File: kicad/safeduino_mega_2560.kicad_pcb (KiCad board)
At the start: 4 copper layers, 134.5 x 63.9 mm, 108 parts, among them X1 USBB-1J

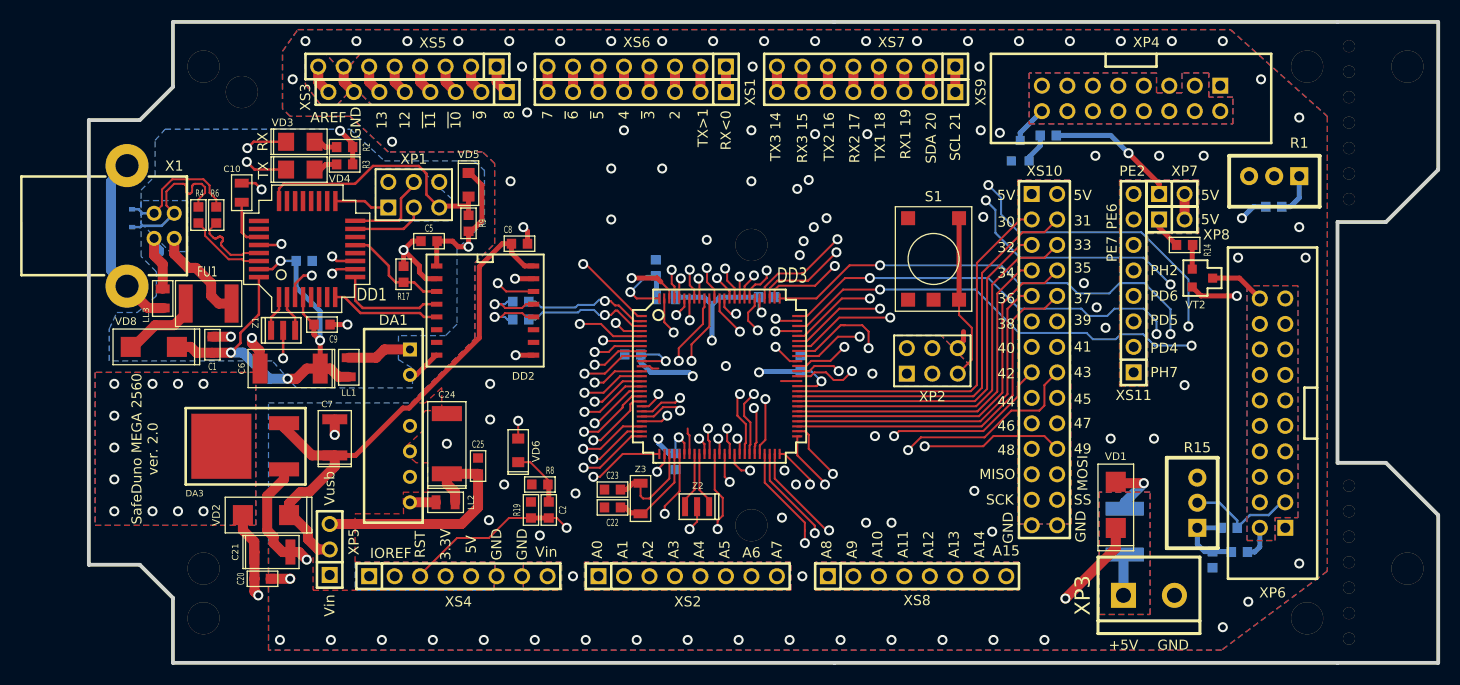
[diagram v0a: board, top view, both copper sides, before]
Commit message: Сохранил проект печатной платы в KiCad 6.0.2. и исправил недочёты в трассировке.
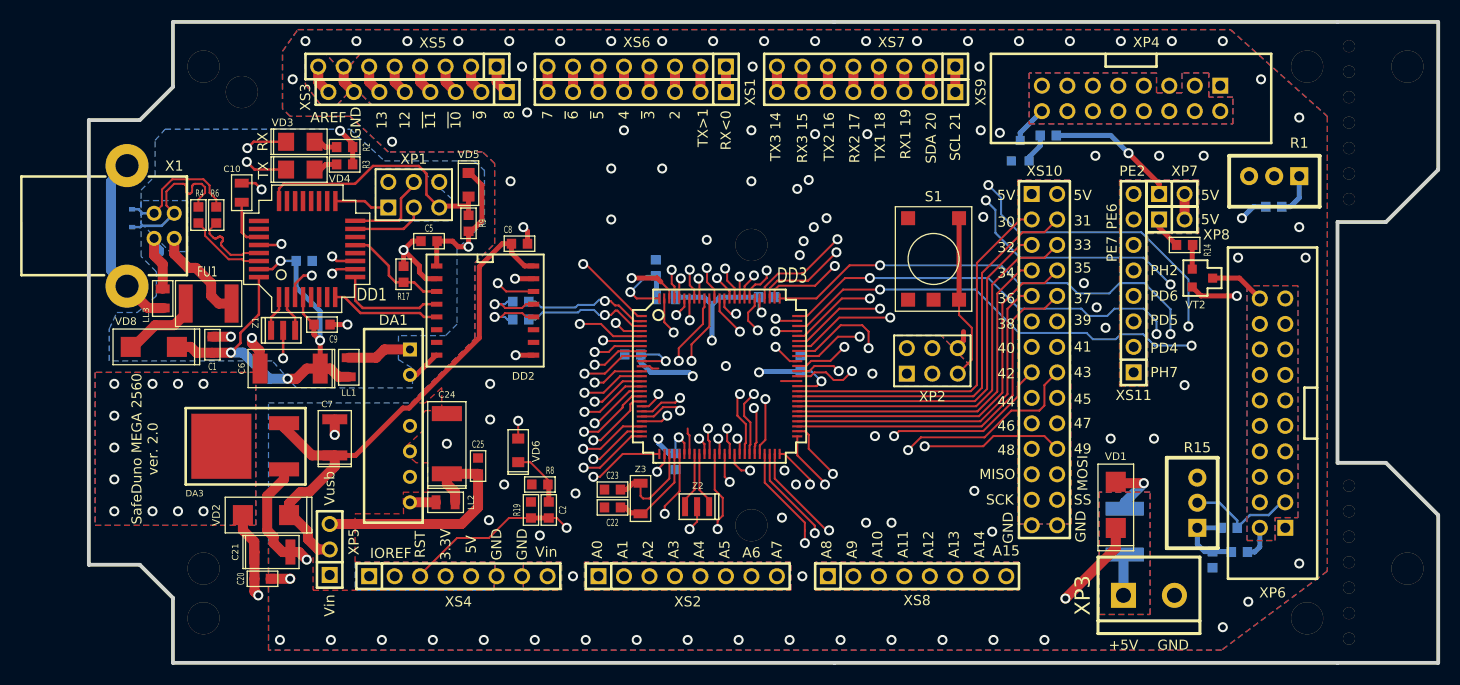
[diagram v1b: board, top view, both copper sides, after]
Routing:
- net /ADC9: track 37.7 -> 33.6 mm
- net /MPU_VCC: track 387.2 -> 383.2 mm
- net /VO_LCD: track 12.6 -> 10.9 mm
- net /GND_USB: track 38.4 -> 36.9 mm
- net /PJ5: track 44.9 -> 43.8 mm
- net /PE7: track 78.9 -> 77.8 mm
- net Net-(R1-Pad2): track 13.5 -> 12.5 mm
- net /5V_USB: track 117.8 -> 116.9 mm
- net /PE6: track 74.8 -> 73.8 mm
- net /PB5: track 56.5 -> 55.7 mm
- net /PD0: track 49.8 -> 49.2 mm
- net /PC3: track 63.1 -> 62.6 mm
- net /PC1: track 69.0 -> 68.4 mm
- net /PH4: track 45.1 -> 44.6 mm
- net /V_OUT: track 19.1 -> 18.6 mm
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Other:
- net class Default removed
- board text added: "~{10}"
- board text added: "~{11}"
- board text added: "~{3}"
- board text added: "~{5}"
- board text added: "~{6}"
- board text added: "~{9}"
- board text removed: "~10"
- board text removed: "~11"
- board text removed: "~3"
- board text removed: "~5"
- board text removed: "~6"
- board text removed: "~9"
